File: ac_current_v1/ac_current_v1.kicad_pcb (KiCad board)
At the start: 2 copper layers, 107.7 x 89.4 mm, 39 parts, among them J1 ICSP, J10 Flow_1, J11 Flow_2, J12 NC_Liquid_1, J13 NC_Liquid_2, J2 UART, J3 AC1_IN, J4 AC1_OUT, J5 AC2_IN, J6 AC2_OUT, J7 GMS1005, SW1 AC_SLCT, SW2 MODE, U1 NRF24L01_Breakout, U2 AMS1117-3.3, U3 ATmega328P-AU, U4 ACS712_1, U5 ACS712_2, Y1 16Mhz

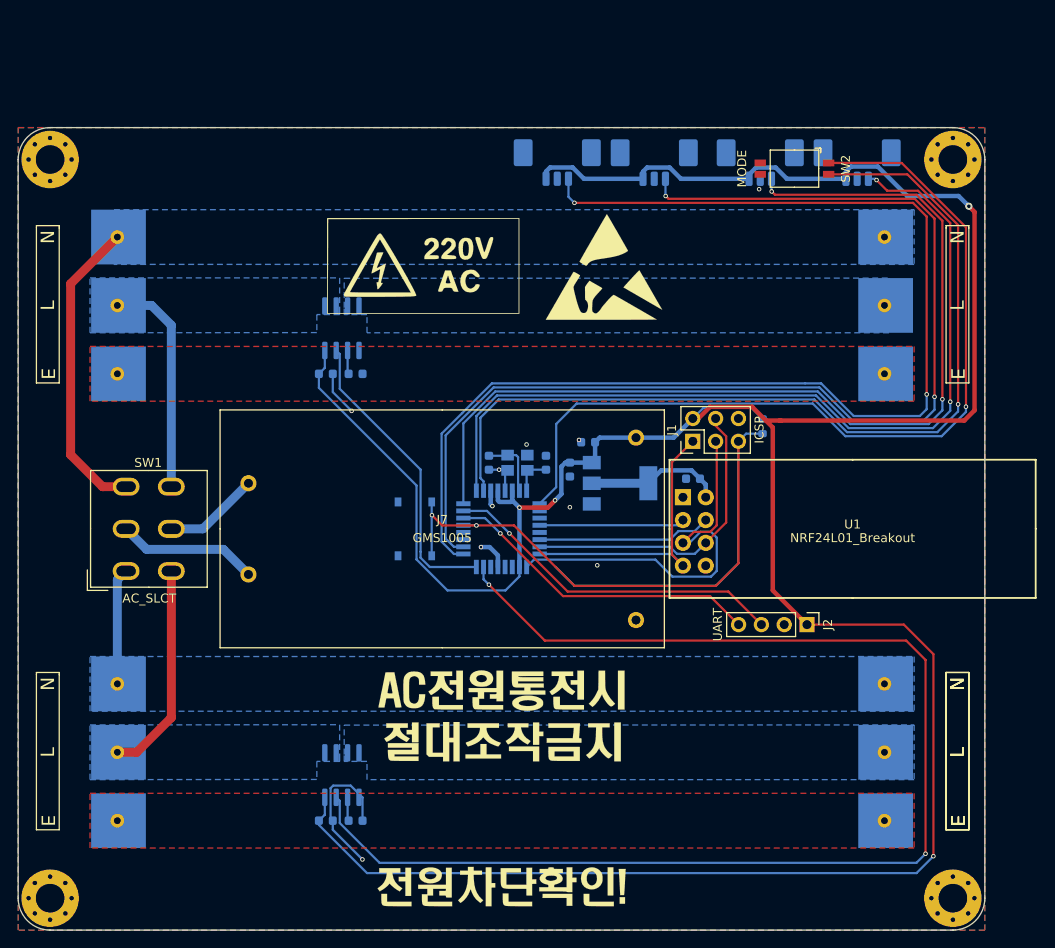
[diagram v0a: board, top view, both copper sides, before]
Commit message: PCB Update
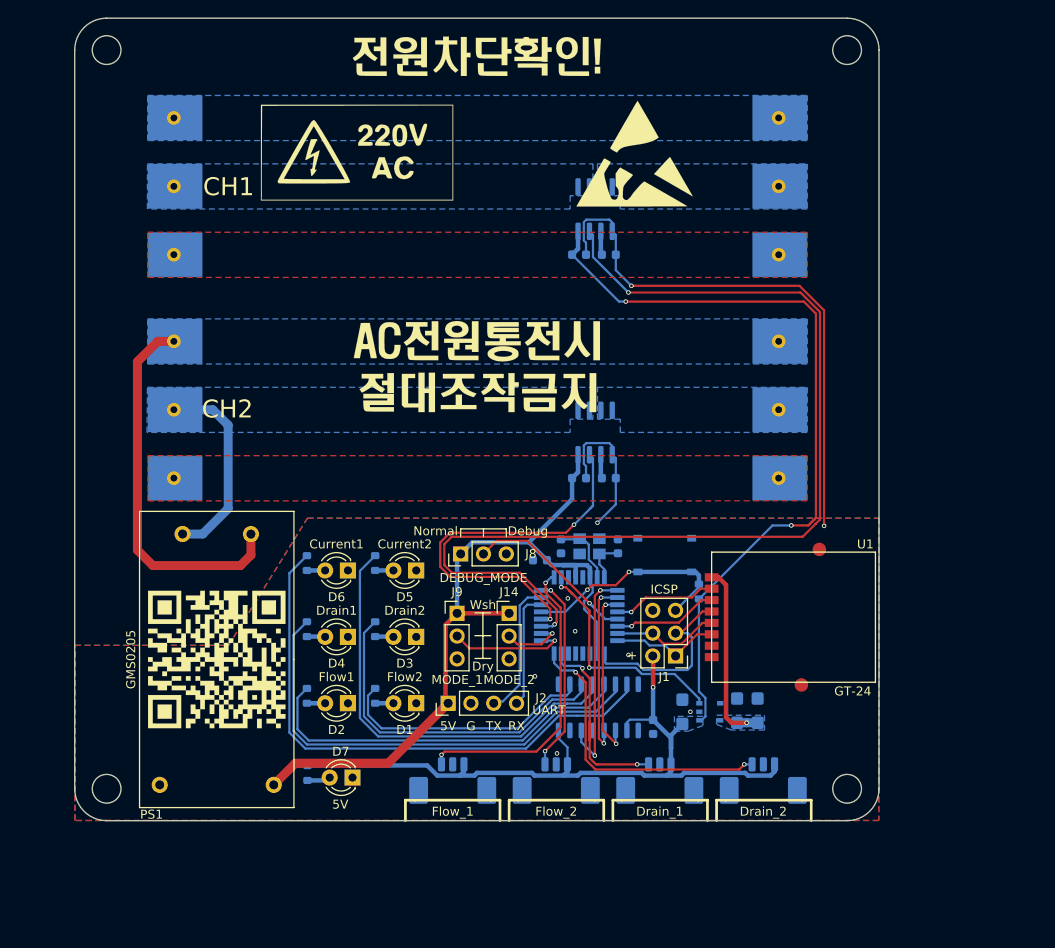
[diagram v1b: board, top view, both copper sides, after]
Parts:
- removed the G*** at (190.4, 100.2)
- removed J7: GMS1005, KIcad:GMS1012
- removed SW1: AC_SLCT, KIcad:MTS-202
- removed SW2: MODE, KIcad:DSHP02TSGER
- added C10: 10uf, Capacitor_Tantalum_SMD:CP_EIA-3216-18_Kemet-A, B.Cu at (178.8, 120.5)
- added C15: 100nf, Capacitor_SMD:C_0603_1608Metric, B.Cu at (167.1, 122.3)
- added D1: Flow2, LED_THT:LED_D3.0mm, F.Cu at (140.7, 119.6)
- added D2: Flow1, LED_THT:LED_D3.0mm, F.Cu at (133.1, 119.6)
- added D3: Drain2, LED_THT:LED_D3.0mm, F.Cu at (140.7, 112.2)
- added D4: Drain1, LED_THT:LED_D3.0mm, F.Cu at (133.1, 112.2)
- added D5: Current2, LED_THT:LED_D3.0mm, F.Cu at (140.7, 104.8)
- added D6: Current1, LED_THT:LED_D3.0mm, F.Cu at (133.1, 104.8)
- added D7: 5V, LED_THT:LED_D3.0mm, F.Cu at (133.6, 127.9)
- added G***: LOGO, KIcad:qrcode, F.Cu at (118.4, 114.7)
- added J14: MODE_2, Connector_PinHeader_2.54mm:PinHeader_1x03_P2.54mm_Vertical, F.Cu at (151.1, 109.6)
- added J8: DEBUG_MODE, Connector_PinHeader_2.54mm:PinHeader_1x03_P2.54mm_Vertical, F.Cu at (145.7, 103.0)
- added J9: MODE_1, Connector_PinHeader_2.54mm:PinHeader_1x03_P2.54mm_Vertical, F.Cu at (145.3, 109.6)
- added PS1: GMS0205, KIcad:GMS0205, F.Cu at (118.5, 114.8)
- added R2: 330, Resistor_SMD:R_0603_1608Metric, B.Cu at (136.2, 118.8)
- added R3: 330, Resistor_SMD:R_0603_1608Metric, B.Cu at (128.6, 118.8)
- added R4: 330, Resistor_SMD:R_0603_1608Metric, B.Cu at (136.2, 111.4)
- added R5: 330, Resistor_SMD:R_0603_1608Metric, B.Cu at (128.6, 111.4)
- added R6: 330, Resistor_SMD:R_0603_1608Metric, B.Cu at (136.2, 104.0)
- added R7: 330, Resistor_SMD:R_0603_1608Metric, B.Cu at (128.6, 104.0)
- added R8: 330, Resistor_SMD:R_0603_1608Metric, B.Cu at (128.6, 127.4)
- added REF**: SMD_762_MountHole, KIcad:SMD_762_MountHole, F.Cu at (105.7, 86.9)
- added REF**: SMD_762_MountHole, KIcad:SMD_762_MountHole, F.Cu at (105.7, 62.0)
- added REF**: SMD_762_MountHole, KIcad:SMD_762_MountHole, F.Cu at (189.0, 86.9)
- added REF**: SMD_762_MountHole, KIcad:SMD_762_MountHole, F.Cu at (189.0, 62.0)
- added U6: 74HC595, Package_SO:SO-16_3.9x9.9mm_P1.27mm, B.Cu at (161.0, 120.1)
- C1, C2: value 100nf -> 10uf; footprint Capacitor_SMD:C_0603_1608Metric -> Capacitor_Tantalum_SMD:CP_EIA-3216-18_Kemet-A
- H1, H2, H3, H4: footprint MountingHole:MountingHole_3.2mm_M3_Pad_Via -> MountingHole:MountingHole_3.2mm_M3
- J12: value NC_Liquid_1 -> Drain_1
- J13: value NC_Liquid_2 -> Drain_2
- J3: value AC1_IN -> AC2_IN
- J4: value AC1_OUT -> AC2_OUT
- J5: value AC2_IN -> AC1_IN
- J6: value AC2_OUT -> AC1_OUT
- R1: value 1k -> 10k
- U1: value NRF24L01_Breakout -> GT-24; footprint KIcad:NRF24L01_PA_LNA -> KIcad:nrf24l01 smd
- U2: value AMS1117-3.3 -> NCP603SN330; footprint Package_TO_SOT_SMD:SOT-223-3_TabPin2 -> Package_SO:TSOP-5_1.65x3.05mm_P0.95mm
- moved G*** 92.5 mm to (147.5, 47.6)
- moved J10 83.3 mm to (144.8, 128.8), turned to 180 degrees
- moved J13 73.7 mm to (179.4, 128.8), turned to 180 degrees
- moved J11 73.6 mm to (156.3, 128.8), turned to 180 degrees
- moved J12 70.0 mm to (167.9, 128.8), turned to 180 degrees
- moved C8 47.5 mm to (158.9, 94.6)
- moved C9 47.5 mm to (162.2, 94.6)
- moved U5 47.5 mm to (160.7, 89.5)
- moved J2 40.9 mm to (144.3, 119.6), turned to 90 degrees
- moved J6 39.9 mm to (181.3, 86.9)
- moved G*** 39.0 mm to (147.5, 82.1)
- moved J5 38.7 mm to (113.9, 86.9)
- moved C1 31.8 mm to (170.4, 120.6), turned to 90 degrees
- moved C6 31.2 mm to (158.9, 69.7)
- moved C7 31.2 mm to (162.2, 69.7)
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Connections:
- net Net-(J5-Pad2) renamed NEUT
- net Net-(J5-Pad3) renamed LINE
- net Net-(U3-Pad19) renamed /A6
- net Net-(U3-Pad22) renamed /A7
- H1 pad 1: GND -> Net-(H1-Pad1)
- H2 pad 1: GND -> Net-(H2-Pad1)
- H3 pad 1: GND -> Net-(H3-Pad1)
- H4 pad 1: GND -> Net-(H4-Pad1)
- J12 pad 3: /A3 -> /A0
- J13 pad 3: /A2 -> /A1
- J3 pad 1: Earth -> GND1
- J4 pad 1: Earth -> GND1
- J5 pad 1: Earth -> GND2
- J6 pad 1: Earth -> GND2
- U1 pad 1: GND -> +3V3
- U1 pad 2: +3V3 -> /D8
- U1 pad 3: /D8 -> /D10
- U1 pad 4: /D10 -> /D13
- U1 pad 5: /D13 -> /D11
- U1 pad 6: /D11 -> /D12
- U1 pad 7: /D12 -> Net-(U1-Pad7)
- U1 pad 8: Net-(U1-Pad8) -> GND
- U2 pad 1: GND -> +5V
- U2 pad 2: +3V3 -> GND
- U2 pad 3: +5V -> /D4
- U4 pad 7: /A1 -> /A4
- U5 pad 7: /A0 -> /A5
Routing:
- net /A2: track 137.5 -> 13.4 mm, vias 2 -> 1
- net /A0: track 146.5 -> 22.9 mm
- net /A3: track 126.7 -> 6.96 mm, vias 2 -> 1
- net /A4: track 0.00 -> 117.2 mm, vias 0 -> 2
- net /D2: track 108.8 -> 22.0 mm
- net /D4: track 102.3 -> 27.5 mm, vias 1 -> 2
- net /RST: track 98.5 -> 24.6 mm
- net +5V: track 337.3 -> 263.8 mm, vias 4 -> 3
- net /D5: track 97.7 -> 24.4 mm, vias 1 -> 2
- net /D3: track 96.5 -> 33.6 mm
- net Net-(R7-Pad1): track 0.00 -> 62.3 mm
- net Net-(R5-Pad1): track 0.00 -> 52.6 mm
- net Net-(R6-Pad1): track 0.00 -> 49.4 mm
- net GND: track 31.1 -> 78.9 mm, vias 10 -> 9
- net /A5: track 0.00 -> 44.1 mm, vias 0 -> 2
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- added copper zone on B.Cu, net +3V3
- added copper zone on B.Cu, net +5V
- added copper zone on F.Cu, net GND1
- added copper zone on F.Cu, net GND2
- removed copper zone on F.Cu, net Earth
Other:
- board size 107.7 x 89.4 mm -> 89.6 x 89.4 mm
- board text added: "+"
- board text added: "5V"
- board text added: "CH1"
- board text added: "CH2"
- board text added: "Debug"
- board text added: "Drain_1"
- board text added: "Drain_2"
- board text added: "Dry"
- board text added: "Flow_1"
- board text added: "Flow_2"
- board text added: "G"
- board text added: "Normal"
- board text added: "RX"
- board text added: "TX"
- board text added: "Wsh"
